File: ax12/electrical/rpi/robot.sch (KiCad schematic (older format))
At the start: 17 parts, among them J1 Raspberry_Pi_2_3, J2 IMU, J3 serial0, J4 I2C, J5 SPI 3V3, J7 Audio, J8 USB SER 3V3, J9 DATA 5V, Q1 BSS138, U2 74LVC1G125, U3 74LVC1G126

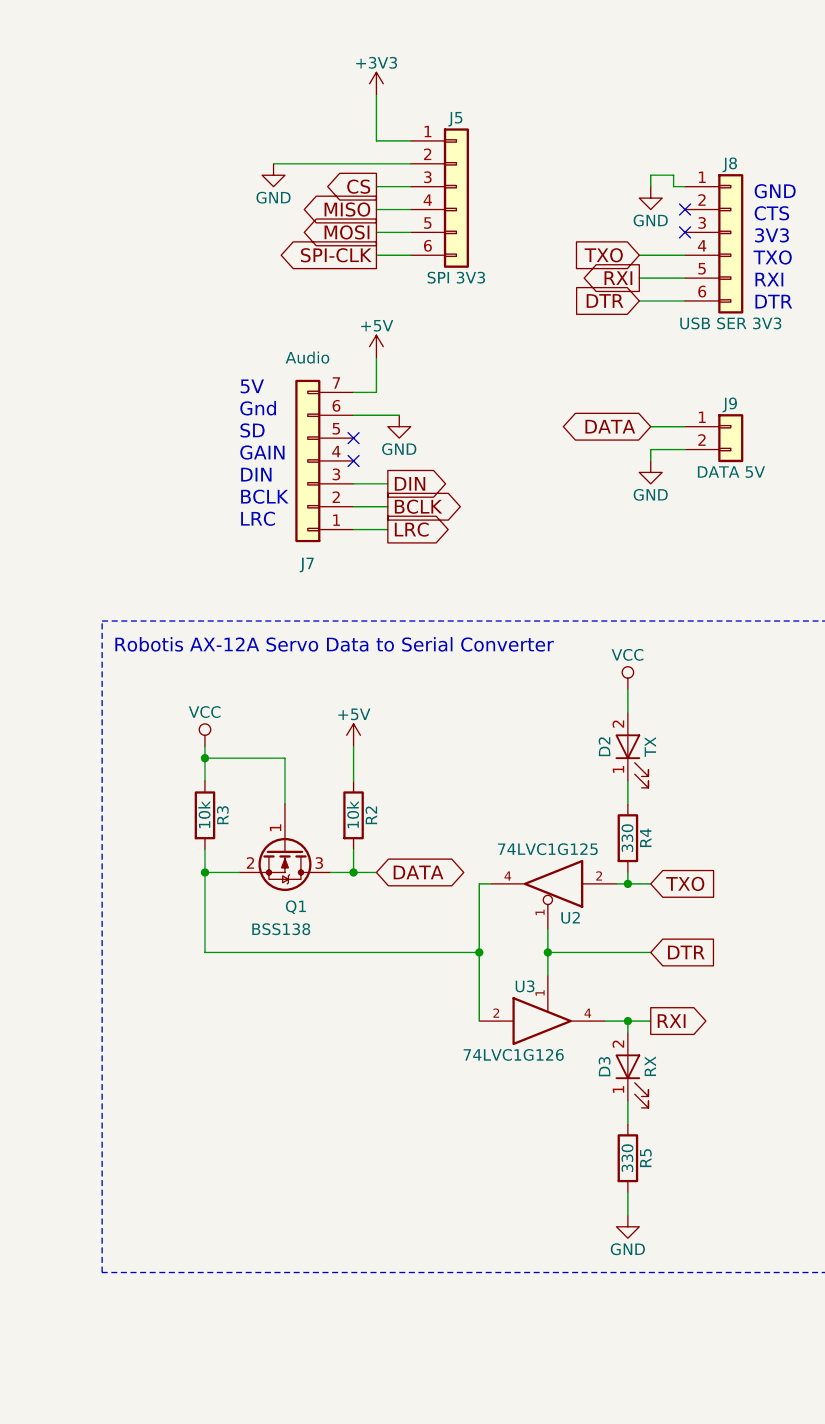
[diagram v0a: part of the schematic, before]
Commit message: power version 5 done and reorg
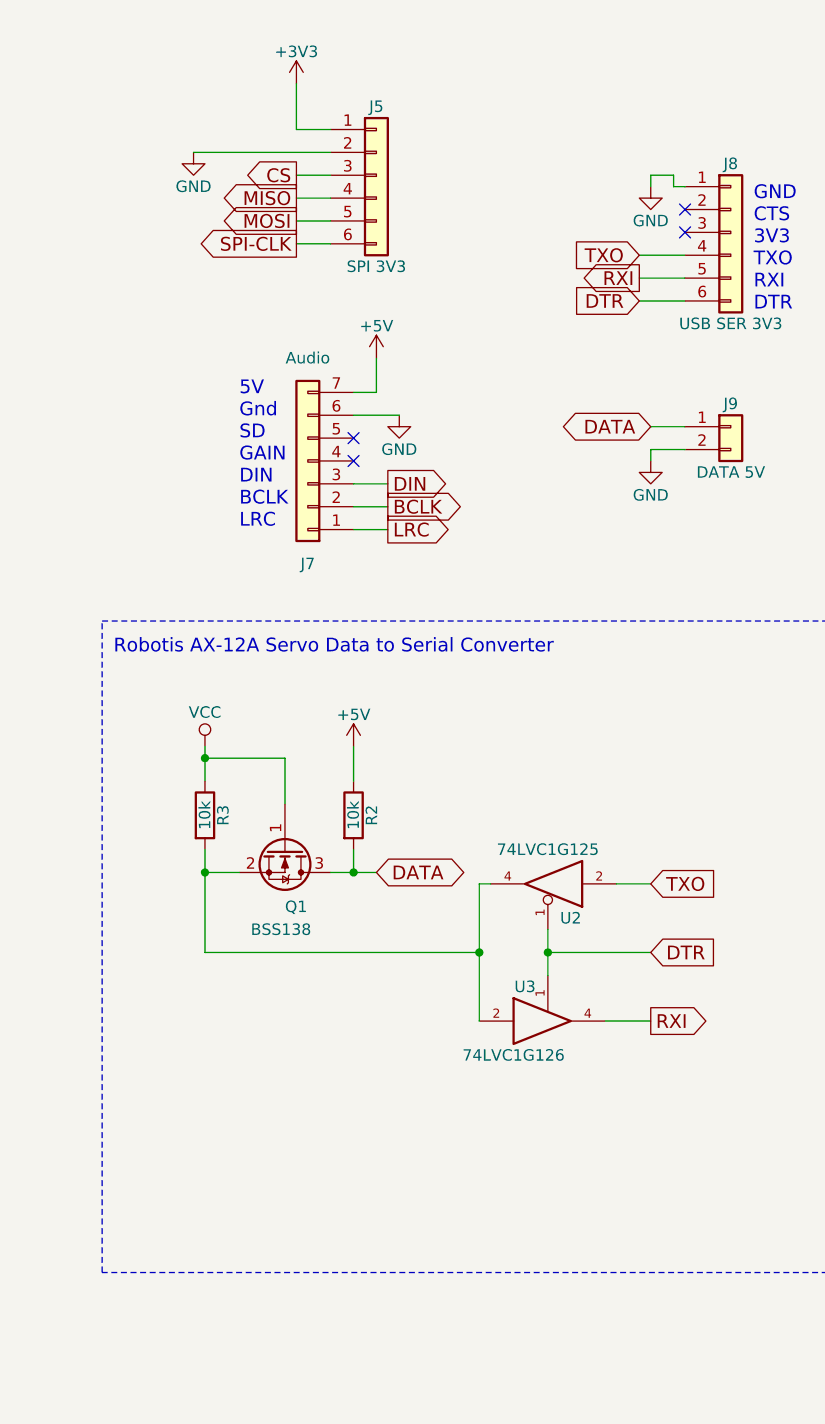
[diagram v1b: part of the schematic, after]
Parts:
- removed D2: TX, LEDs:LED_1206_HandSoldering, symbol LED
- removed D3: RX, LEDs:LED_1206_HandSoldering, symbol LED
- removed R4, R5: 330, Resistors_SMD:R_1206_HandSoldering, symbol R
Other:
- moved on the sheet: J5
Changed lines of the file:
@@
 Text GLabel 4600 2850 2    60   Output ~ 0
 CS
-Text GLabel 8550 1400 0    60   Output ~ 0
+Text GLabel 8200 1350 0    60   Output ~ 0
 CS
 Text GLabel 4600 3050 2    60   Output ~ 0
@@
 Text GLabel 4600 2950 2    60   Output ~ 0
 MISO
-Text GLabel 8550 1600 0    60   Output ~ 0
+Text GLabel 8200 1550 0    60   Output ~ 0
 MOSI
-Text GLabel 8550 1500 0    60   Output ~ 0
+Text GLabel 8200 1450 0    60   Output ~ 0
 MISO
 Text GLabel 4600 3150 2    60   Output ~ 0
 SPI-CLK
-Text GLabel 8550 1700 0    60   Output ~ 0
+Text GLabel 8200 1650 0    60   Output ~ 0
 SPI-CLK
 $Comp
 L Conn_01x06 J5
 U 1 1 5AA22432
-P 8900 1400
-F 0 "J5" H 8900 1700 50  0000 C CNN
-F 1 "SPI 3V3" H 8900 1000 50  0000 C CNN
-F 2 "Pin_Headers:Pin_Header_Straight_1x06_Pitch2.54mm" H 8900 1400 50  0001 C CNN
-F 3 "" H 8900 1400 50  0001 C CNN
-	1    8900 1400
+P 8550 1350
+F 0 "J5" H 8550 1650 50  0000 C CNN
+F 1 "SPI 3V3" H 8550 950 50  0000 C CNN
+F 2 "Pin_Headers:Pin_Header_Straight_1x06_Pitch2.54mm" H 8550 1350 50  0001 C CNN
+F 3 "" H 8550 1350 50  0001 C CNN
+	1    8550 1350
 	1    0    0    -1
 $EndComp
@@
 L +3V3 #PWR013
 U 1 1 5AA22A0F
-P 8550 1000
-F 0 "#PWR013" H 8550 850 50  0001 C CNN
-F 1 "+3V3" H 8550 1140 50  0000 C CNN
-F 2 "" H 8550 1000 50  0001 C CNN
-F 3 "" H 8550 1000 50  0001 C CNN
-	1    8550 1000
+P 8200 950
+F 0 "#PWR013" H 8200 800 50  0001 C CNN
+F 1 "+3V3" H 8200 1090 50  0000 C CNN
+F 2 "" H 8200 950 50  0001 C CNN
+F 3 "" H 8200 950 50  0001 C CNN
+	1    8200 950
 	1    0    0    -1
 $EndComp
@@
 L GND #PWR014
 U 1 1 5AA22A3E
-P 8100 1300
-F 0 "#PWR014" H 8100 1050 50  0001 C CNN
-F 1 "GND" H 8100 1150 50  0000 C CNN
-F 2 "" H 8100 1300 50  0001 C CNN
-F 3 "" H 8100 1300 50  0001 C CNN
-	1    8100 1300
+P 7750 1250
+F 0 "#PWR014" H 7750 1000 50  0001 C CNN
+F 1 "GND" H 7750 1100 50  0000 C CNN
+F 2 "" H 7750 1250 50  0001 C CNN
+F 3 "" H 7750 1250 50  0001 C CNN
+	1    7750 1250
 	1    0    0    -1
 $EndComp
@@
 $EndComp
 $Comp
-L LED D2
-U 1 1 5AA2F8B2
-P 9650 3850
-F 0 "D2" H 9650 3950 50  0000 C CNN
-F 1 "TX" H 9650 3750 50  0000 C CNN
-F 2 "LEDs:LED_1206_HandSoldering" H 9650 3850 50  0001 C CNN
-F 3 "" H 9650 3850 50  0001 C CNN
-	1    9650 3850
-	0    -1   -1   0
-$EndComp
-$Comp
-L LED D3
-U 1 1 5AA2F96E
-P 9650 5250
-F 0 "D3" H 9650 5350 50  0000 C CNN
-F 1 "RX" H 9650 5150 50  0000 C CNN
-F 2 "LEDs:LED_1206_HandSoldering" H 9650 5250 50  0001 C CNN
-F 3 "" H 9650 5250 50  0001 C CNN
-	1    9650 5250
-	0    -1   -1   0
-$EndComp
-$Comp
-L R R4
-U 1 1 5AA2FA9D
-P 9650 4250
-F 0 "R4" V 9730 4250 50  0000 C CNN
-F 1 "330" V 9650 4250 50  0000 C CNN
-F 2 "Resistors_SMD:R_1206_HandSoldering" V 9580 4250 50  0001 C CNN
-F 3 "" H 9650 4250 50  0001 C CNN
-	1    9650 4250
-	1    0    0    -1
-$EndComp
-$Comp
-L R R5
-U 1 1 5AA2FB65
-P 9650 5650
-F 0 "R5" V 9730 5650 50  0000 C CNN
-F 1 "330" V 9650 5650 50  0000 C CNN
-F 2 "Resistors_SMD:R_1206_HandSoldering" V 9580 5650 50  0001 C CNN
-F 3 "" H 9650 5650 50  0001 C CNN
-	1    9650 5650
-	1    0    0    -1
-$EndComp
-$Comp
-L GND #PWR020
-U 1 1 5AA2FDB7
-P 9650 5900
-F 0 "#PWR020" H 9650 5650 50  0001 C CNN
-F 1 "GND" H 9650 5750 50  0000 C CNN
-F 2 "" H 9650 5900 50  0001 C CNN
-F 3 "" H 9650 5900 50  0001 C CNN
-	1    9650 5900
-	1    0    0    -1
-$EndComp
-$Comp
 L Conn_01x06 J8
 U 1 1 5AA30710
@@
 	5400 1950 5600 1950
 Wire Wire Line
-	8700 1300 8100 1300
-Wire Wire Line
-	8700 1200 8550 1200
-Wire Wire Line
-	8550 1200 8550 1000
-Wire Wire Line
-	8700 1700 8550 1700
-Wire Wire Line
-	8700 1600 8550 1600
-Wire Wire Line
-	8700 1500 8550 1500
-Wire Wire Line
-	8700 1400 8550 1400
+	8350 1250 7750 1250
+Wire Wire Line
+	8350 1150 8200 1150
+Wire Wire Line
+	8200 1150 8200 950
+Wire Wire Line
+	8350 1650 8200 1650
+Wire Wire Line
+	8350 1550 8200 1550
+Wire Wire Line
+	8350 1450 8200 1450
+Wire Wire Line
+	8350 1350 8200 1350
 Wire Wire Line
 	9600 4450 9750 4450
@@
 Wire Notes Line
 	10650 6150 7350 6150
-Wire Wire Line
-	9650 3600 9650 3700
-Wire Wire Line
-	9650 4000 9650 4100
-Wire Wire Line
-	9650 4400 9650 4450
-Connection ~ 9650 4450
-Wire Wire Line
-	9650 5100 9650 5050
-Connection ~ 9650 5050
-Wire Wire Line
-	9650 5500 9650 5400
-Wire Wire Line
-	9650 5900 9650 5800
 Wire Wire Line
 	9900 1400 9850 1400
@@
 	1    0    0    -1
 $EndComp
-$Comp
-L VCC #PWR?
-U 1 1 5AAD9DC7
-P 9650 3600
-F 0 "#PWR?" H 9650 3450 50  0001 C CNN
-F 1 "VCC" H 9650 3750 50  0000 C CNN
-F 2 "" H 9650 3600 50  0001 C CNN
-F 3 "" H 9650 3600 50  0001 C CNN
-	1    9650 3600
-	1    0    0    -1
-$EndComp
